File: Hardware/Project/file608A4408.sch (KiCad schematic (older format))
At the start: 36 parts, among them Q3 Q_PNP_BCE, Q4 Q_PNP_BCE, Q5 Q_PNP_BCE, Q6 Q_PNP_BCE, Q7 Q_PNP_BCE, Q8 Q_PNP_BCE

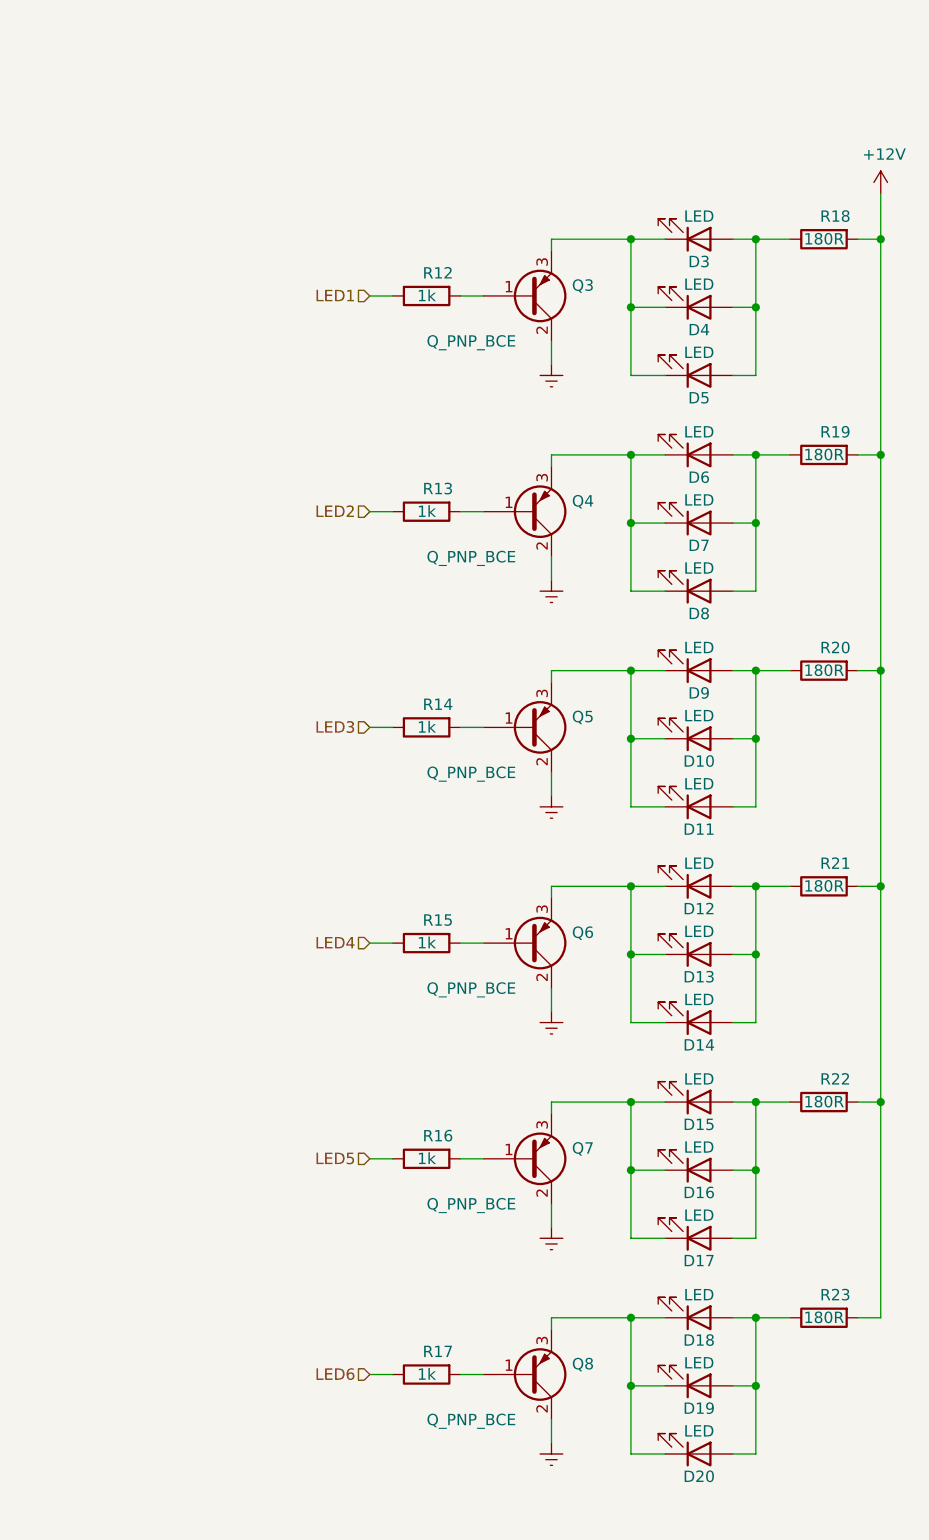
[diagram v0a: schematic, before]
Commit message: update 21-03-21
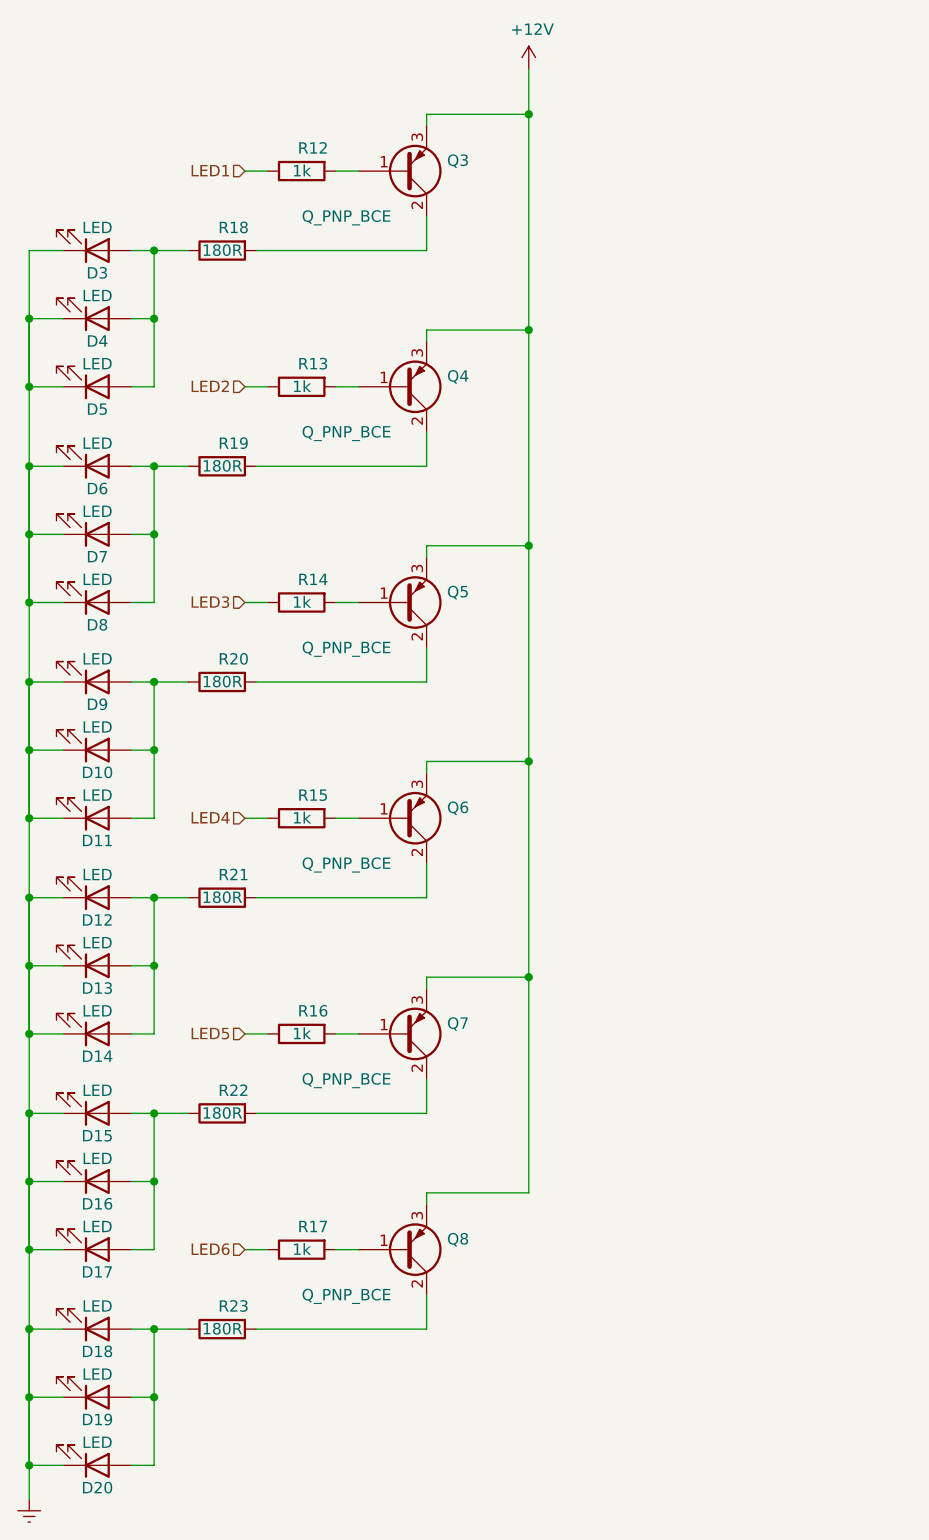
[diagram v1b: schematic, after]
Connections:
- net +12V: now also Q3.3 (E), Q4.3 (E), Q5.3 (E), Q6.3 (E), Q7.3 (E), Q8.3 (E); no longer R18.2, R19.2, R20.2, R21.2, R22.2, R23.2
- net Earth: now also D10.1 (K), D11.1 (K), D12.1 (K), D13.1 (K), D14.1 (K), D15.1 (K), D16.1 (K), D17.1 (K), D18.1 (K), D19.1 (K), D20.1 (K), D3.1 (K), D4.1 (K), D5.1 (K), D6.1 (K), D7.1 (K), D8.1 (K), D9.1 (K); no longer Q3.2 (C), Q4.2 (C), Q5.2 (C), Q6.2 (C), Q7.2 (C), Q8.2 (C)
- new net: Q3.2 (C), R18.2
- new net: Q4.2 (C), R19.2
- new net: Q5.2 (C), R20.2
- new net: Q6.2 (C), R21.2
- new net: Q7.2 (C), R22.2
- new net: Q8.2 (C), R23.2
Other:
- moved on the sheet: D10, D11, D12, D13, D14, D15, D16, D17, D18, D19, D20, D3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
